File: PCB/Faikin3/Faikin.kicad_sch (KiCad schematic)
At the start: 37 parts, among them J1 1x5, J2 Prog, Q3 PMF250XNEX, U1 ESP32-PICO-MINI-02, U2 Barcode, U3 MD8942, U4 Barcode

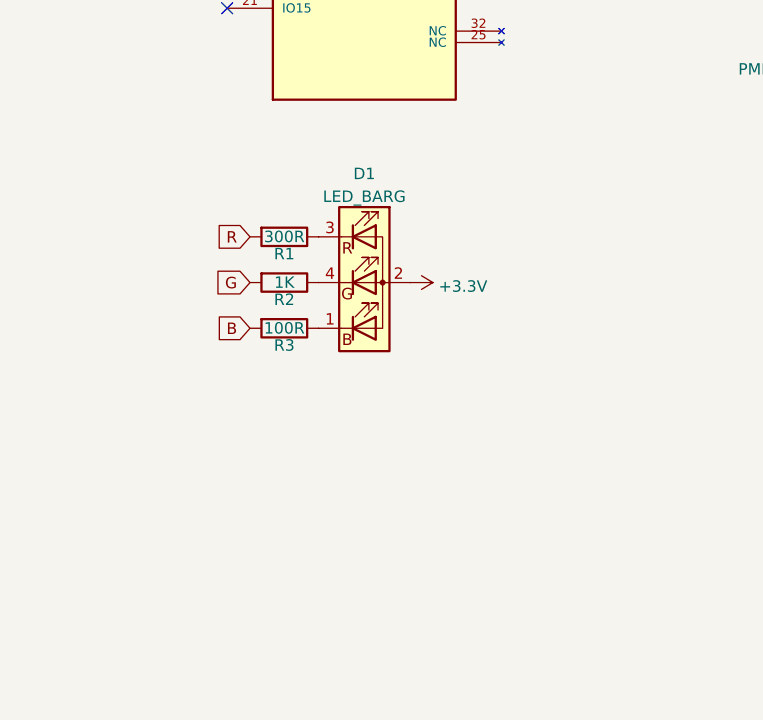
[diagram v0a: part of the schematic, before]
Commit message: tidy, new LED
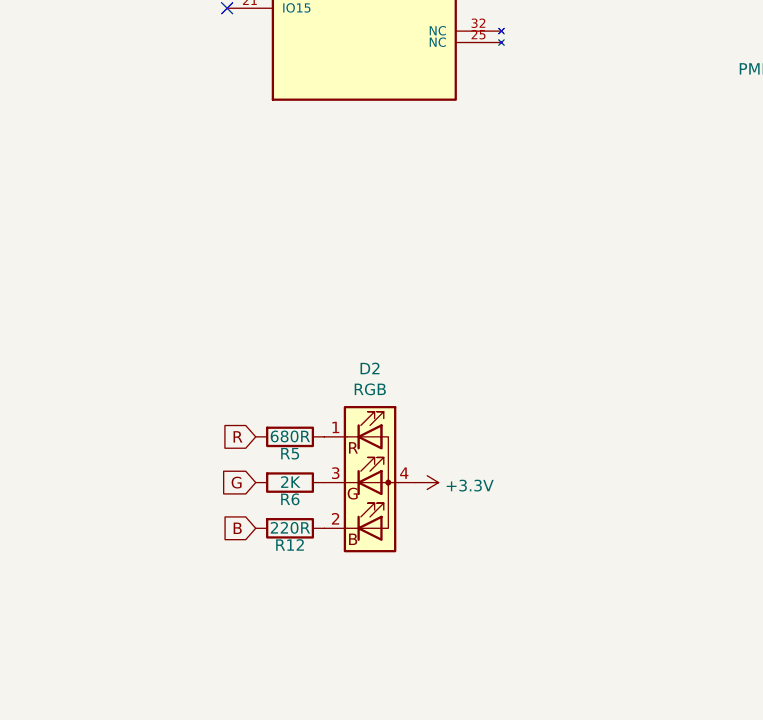
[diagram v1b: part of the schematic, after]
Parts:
- removed D1: LED_BARG, RevK:MHS190RGBCT, symbol Device:LED_BARG
- removed R1: 300R, RevK:R_0402, symbol Device:R
- removed R2: 1K, RevK:R_0402, symbol Device:R
- removed R3: 100R, RevK:R_0402, symbol Device:R
- added D2: RGB, RevK:LED-RGB-1.6x1.6, symbol Device:LED_RBGA
- added R12: 220R, RevK:R_0402, symbol Device:R
- added R5: 680R, RevK:R_0402, symbol Device:R
- added R6: 2K, RevK:R_0402, symbol Device:R
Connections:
- net +3.3V: now also D2.4 (A)
- net B: now also R12.2
- net G: now also R6.2
- net R: now also R5.2
- new net: D2.2 (BK), R12.1
- new net: D2.1 (RK), R5.1
- new net: D2.3 (GK), R6.1
